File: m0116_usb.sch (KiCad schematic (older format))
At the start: 186 parts, among them J1 USB_C_port, J2 Conn_01x04, J3 Conn_01x04, J4 AVR-ISP-6, K1 ESC, K10 9, K11 0, K12 -, K13 =, K14 backspace, K15 num_clear, K16 =, K17 /, K18 *, K19 tab, K2 1, K20 Q, K21 W, K22 E, K23 R, K24 T, K25 Y, K26 U, K27 I, K28 O, K29 P, K3 2, K30 [, K31 ], K32 enter, K33 num_7, K34 num_8, K35 num_9, K36 +, K37 control, K38 A, K39 S, K4 3, K40 D, K41 F, K42 G, K43 H, K44 J, K45 K, K46 L, K47 ;, K48 ', K49 num_4, K5 4, K50 num_5, K51 num_6, K52 -, K53 shift, K54 Z, K55 X, K56 C, K57 V, K58 B, K59 N, K6 5, K60 M, K61 ,, K62 ., K63 /, K64 r_shift, K65 num_1, K66 num_2, K67 num_3, K68 capslock, K69 option, K7 6, K70 mac, K72 long_sw, K73 space, K74 \\, K75 left, K76 right, K77 down, K78 up, K79 num_0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

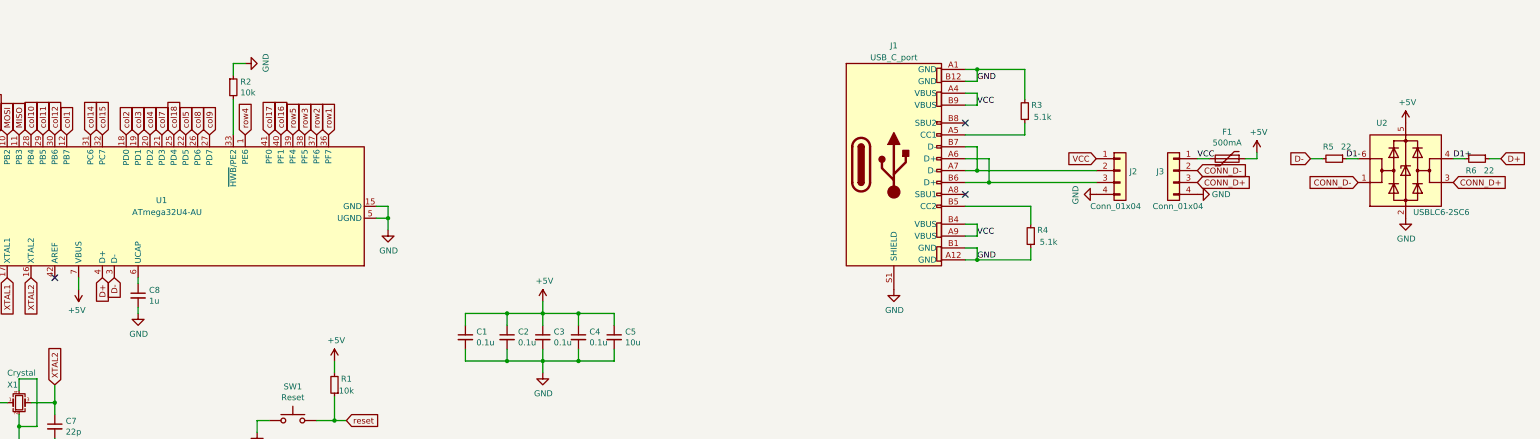
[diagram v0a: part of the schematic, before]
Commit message: revise daughterboard, finalize
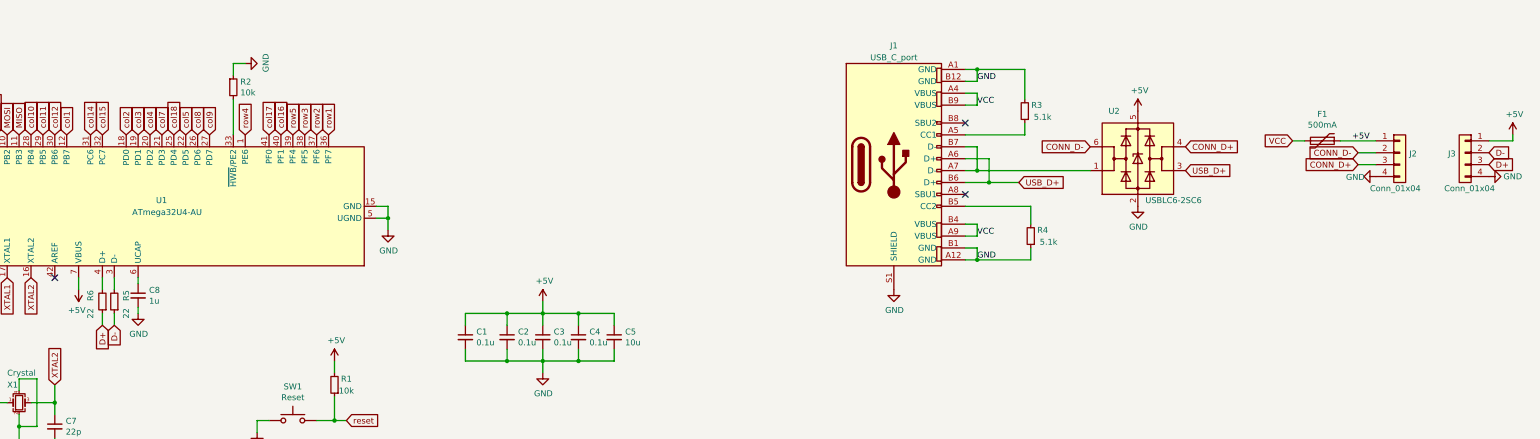
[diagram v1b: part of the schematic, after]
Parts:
- C1, C2, C3, C4: LCSC Part # (none) -> C14663; LCSC Part Number (none) -> C14663
- C5: LCSC Part # (none) -> C19702; LCSC Part Number (none) -> C19702
- C6, C7: LCSC Part # (none) -> C1555; LCSC Part Number (none) -> C1555
- C8: LCSC Part # (none) -> C52923; LCSC Part Number (none) -> C52923
- D1, D10, D11, D12, D13, D14, D15, D16, D17, D18, D19, D2, D20, D21, D22, D23, D24, D25, D26, D27, D28, D29, D3, D30, D31, D32, D33, D34, D35, D36, D37, D38, D39, D4, D40, D41, D42, D43, D44, D45, D46, D47, D48, D49, D5, D50, D51, D52, D53, D54, D55, D56, D57, D58, D59, D6, D60, D61, D62, D63, D64, D65, D66, D67, D68, D69, D7, D70, D71, D72, D73, D74, D75, D76, D77, D78, D79, D8, D80, D81, D9: LCSC Part # (none) -> C81598; LCSC Part Number (none) -> C81598
- F1: LCSC Part # (none) -> C135336; LCSC Part Number (none) -> C135336
- J1: LCSC Part # (none) -> C393939; LCSC Part Number (none) -> C393939
- J3: LCSC Part # (none) -> C239522; LCSC Part Number (none) -> C239522
- R1, R2: LCSC Part # (none) -> C25197; LCSC Part Number (none) -> C25197
- R3, R4: LCSC Part # (none) -> C23186; LCSC Part Number (none) -> C23186
- R5, R6: LCSC Part # (none) -> C23345; LCSC Part Number (none) -> C23345
- SW1: LCSC Part # (none) -> C318884; LCSC Part Number (none) -> C318884
- SW2: footprint Button_Switch_SMD:SW_SPDT_CK-JS102011SAQN -> project_custom_parts:SW_SPDT_SK-3245S-L1-A; LCSC Part # (none) -> C405951; LCSC Part Number (none) -> C405951
- U1: LCSC Part # (none) -> C44854; LCSC Part Number (none) -> C44854
- U2: LCSC Part # (none) -> C2687116; LCSC Part Number (none) -> C2687116
- X1: LCSC Part # (none) -> C160456; LCSC Part Number (none) -> C160456
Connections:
- net +5V: now also J2.1 (Pin_1), J3.1 (Pin_1)
- net CONN_D+: now also J2.3 (Pin_3), U2.4 (I/O2); no longer J3.3 (Pin_3), U2.3 (I/O2)
- net CONN_D-: now also J2.2 (Pin_2), U2.6 (I/O1); no longer J3.2 (Pin_2), U2.1 (I/O1)
- net D+: now also J3.3 (Pin_3); no longer U1.4 (D+)
- net D-: now also J3.2 (Pin_2), R5.1; no longer R5.2, U1.3 (D-)
- net VCC: no longer J2.1 (Pin_1), J3.1 (Pin_1)
- net at J1.A7 (D-), J1.B7 (D-): now also U2.1 (I/O1); no longer J2.2 (Pin_2)
- net USB_D+: now reaches J1.A6 (D+), J1.B6 (D+)
- net USB_D+: now also U2.3 (I/O2); no longer J2.3 (Pin_3)
- net D1+: no longer names the net of R6.2
- net D1+: now also U1.4 (D+); no longer U2.4 (I/O2)
- removed net D1-: R5.1, U2.6 (I/O1)
- new net: R5.2, U1.3 (D-)
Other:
- moved on the sheet: F1, J2, J3, R5, R6, U2
